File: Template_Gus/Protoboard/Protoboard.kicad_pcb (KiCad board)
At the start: 2 copper layers, 247 x 81.3 mm, 2 parts

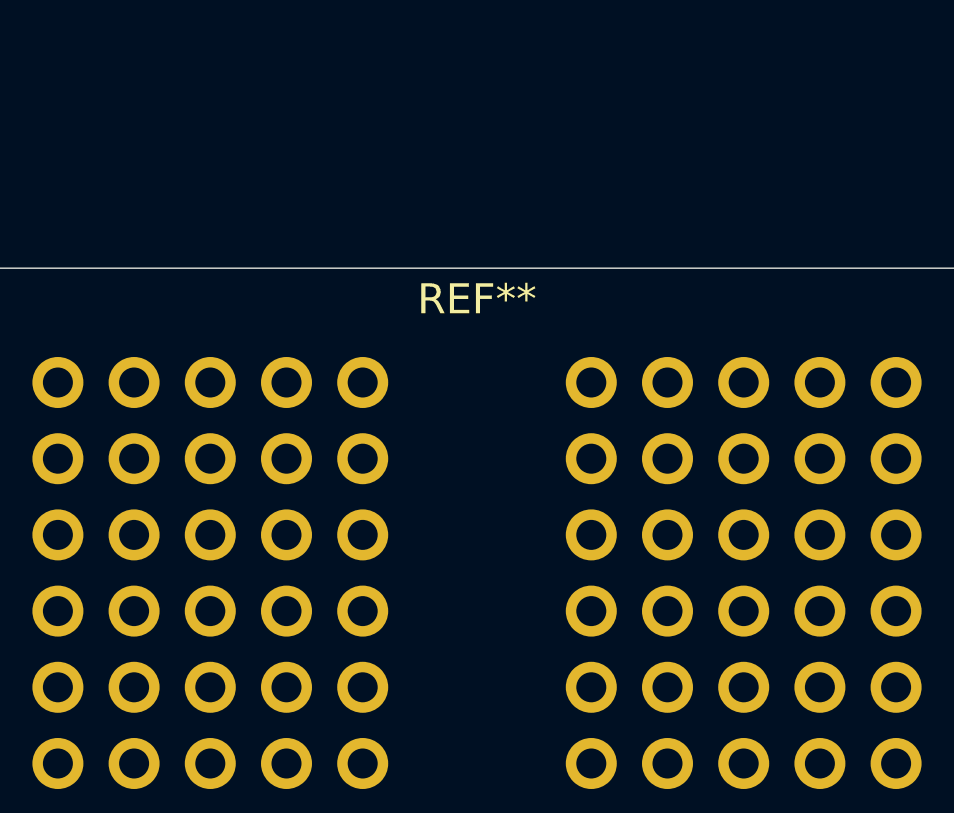
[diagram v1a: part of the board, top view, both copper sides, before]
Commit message: Add the Key
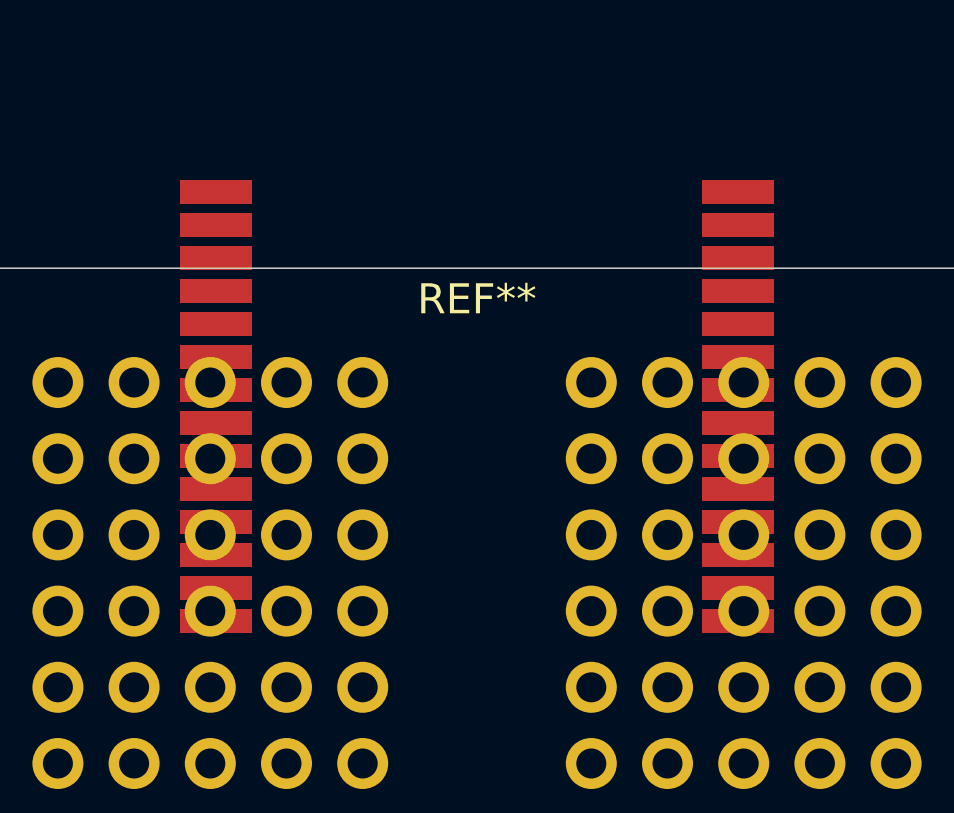
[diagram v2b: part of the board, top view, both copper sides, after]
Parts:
- added REF**: MS88SF2, Nordic_Module:MS88SF2, F.Cu at (49.5, 61.0)
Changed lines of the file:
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@@
     (tracks 0)
     (zones 0)
-    (modules 2)
+    (modules 3)
     (nets 1)
   )
@@
     (uvia_drill 0.1)
   )
+  (module Nordic_Module:MS88SF2 (layer F.Cu)
+    (at 49.53 60.96)
+    (fp_text reference REF** (at 0 -16.51) (layer F.Fab) hide
+      (effects (font (size 1 1) (thickness 0.15)))
+    )
+    (fp_text value MS88SF2 (at 0 10.795) (layer F.Fab) hide
+      (effects (font (size 1 1) (thickness 0.15)))
+    )
+    (fp_line (start -8.7 8.6868) (end 8.7 8.6868) (layer F.Fab) (width 0.12))
+    (fp_line (start -8.7 8.6868) (end -8.7 -14.5132) (layer F.Fab) (width 0.12))
+    (fp_line (start 8.7 8.6868) (end 8.7 -14.5132) (layer F.Fab) (width 0.12))
+    (fp_line (start -8.7 -14.5132) (end 8.7 -14.5132) (layer F.Fab) (width 0.12))
+    (fp_line (start -8.6868 -7.62) (end 8.6868 -7.62) (layer F.Fab) (width 0.12))
+    (fp_line (start 8.6868 -7.62) (end -8.6868 -14.5034) (layer F.Fab) (width 0.12))
+    (fp_line (start 8.6868 -14.5034) (end -8.6868 -7.62) (layer F.Fab) (width 0.12))
+    (pad 1 smd rect (at -8.7 -6.985) (size 2.4 0.8) (layers F.Cu F.Paste F.Mask))
+    (pad 2 smd rect (at -8.7 -5.885) (size 2.4 0.8) (layers F.Cu F.Paste F.Mask))
+    (pad 3 smd rect (at -8.7 -4.785) (size 2.4 0.8) (layers F.Cu F.Paste F.Mask))
+    (pad 4 smd rect (at -8.7 -3.685) (size 2.4 0.8) (layers F.Cu F.Paste F.Mask))
+    (pad 5 smd rect (at -8.7 -2.585) (size 2.4 0.8) (layers F.Cu F.Paste F.Mask))
+    (pad 6 smd rect (at -8.7 -1.485) (size 2.4 0.8) (layers F.Cu F.Paste F.Mask))
+    (pad 7 smd rect (at -8.7 -0.385) (size 2.4 0.8) (layers F.Cu F.Paste F.Mask))
+    (pad 8 smd rect (at -8.7 0.715) (size 2.4 0.8) (layers F.Cu F.Paste F.Mask))
+    (pad 9 smd rect (at -8.7 1.815) (size 2.4 0.8) (layers F.Cu F.Paste F.Mask))
+    (pad 10 smd rect (at -8.7 2.915) (size 2.4 0.8) (layers F.Cu F.Paste F.Mask))
+    (pad 11 smd rect (at -8.7 4.015) (size 2.4 0.8) (layers F.Cu F.Paste F.Mask))
+    (pad 12 smd rect (at -8.7 5.115) (size 2.4 0.8) (layers F.Cu F.Paste F.Mask))
+    (pad 13 smd rect (at -8.7 6.215) (size 2.4 0.8) (layers F.Cu F.Paste F.Mask))
+    (pad 14 smd rect (at -8.7 7.315) (size 2.4 0.8) (layers F.Cu F.Paste F.Mask))
+    (pad 28 smd rect (at 8.7 -6.985) (size 2.4 0.8) (layers F.Cu F.Paste F.Mask))
+    (pad 27 smd rect (at 8.7 -5.885) (size 2.4 0.8) (layers F.Cu F.Paste F.Mask))
+    (pad 26 smd rect (at 8.7 -4.785) (size 2.4 0.8) (layers F.Cu F.Paste F.Mask))
+    (pad 25 smd rect (at 8.7 -3.685) (size 2.4 0.8) (layers F.Cu F.Paste F.Mask))
+    (pad 24 smd rect (at 8.7 -2.585) (size 2.4 0.8) (layers F.Cu F.Paste F.Mask))
+    (pad 23 smd rect (at 8.7 -1.485) (size 2.4 0.8) (layers F.Cu F.Paste F.Mask))
+    (pad 22 smd rect (at 8.7 -0.385) (size 2.4 0.8) (layers F.Cu F.Paste F.Mask))
+    (pad 21 smd rect (at 8.7 0.715) (size 2.4 0.8) (layers F.Cu F.Paste F.Mask))
+    (pad 20 smd rect (at 8.7 1.815) (size 2.4 0.8) (layers F.Cu F.Paste F.Mask))
+    (pad 19 smd rect (at 8.7 2.915) (size 2.4 0.8) (layers F.Cu F.Paste F.Mask))
+    (pad 18 smd rect (at 8.7 4.015) (size 2.4 0.8) (layers F.Cu F.Paste F.Mask))
+    (pad 17 smd rect (at 8.7 5.115) (size 2.4 0.8) (layers F.Cu F.Paste F.Mask))
+    (pad 16 smd rect (at 8.7 6.215) (size 2.4 0.8) (layers F.Cu F.Paste F.Mask))
+    (pad 15 smd rect (at 8.7 7.315) (size 2.4 0.8) (layers F.Cu F.Paste F.Mask))
+  )
   (module Protoboard:Breadboard_Friendly_Template_800 (layer F.Cu)

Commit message: update
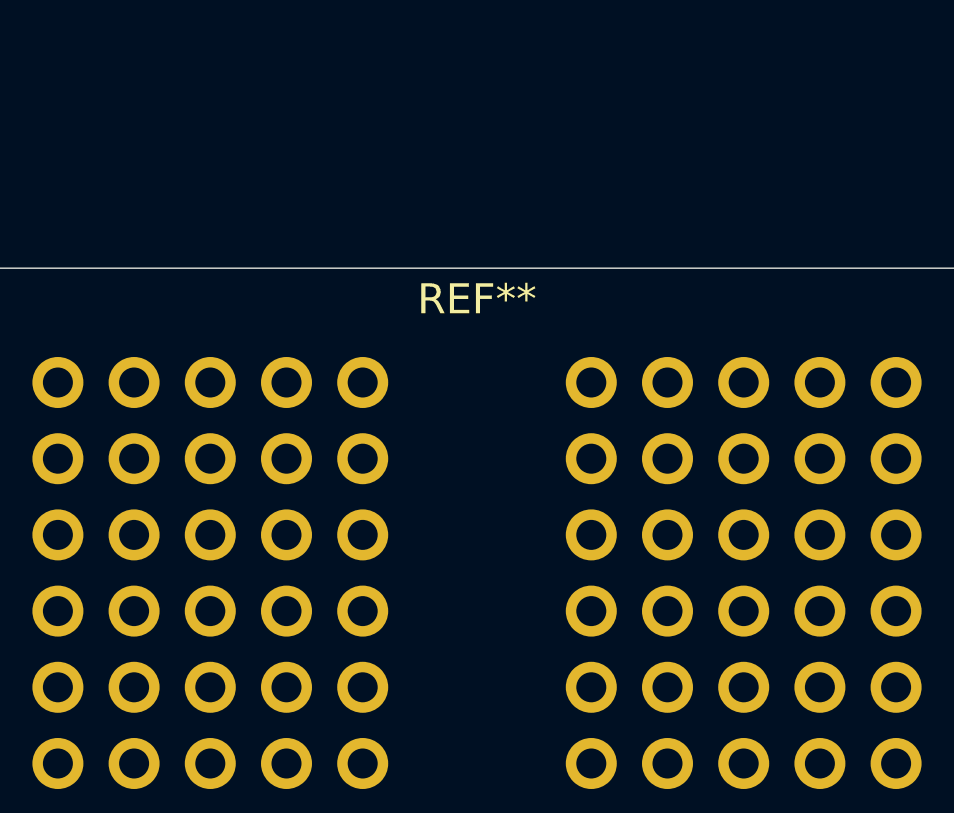
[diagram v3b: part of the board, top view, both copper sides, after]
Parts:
- removed the REF** at (49.5, 61.0)
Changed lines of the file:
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@@
-(kicad_pcb (version 20171130) (host pcbnew 5.1.5-52549c5~84~ubuntu18.04.1)
+(kicad_pcb (version 20171130) (host pcbnew "(5.1.9-0-10_14)")
   (general
     (thickness 1.6)
-    (drawings 33)
+    (drawings 37)
     (tracks 0)
     (zones 0)
-    (modules 3)
+    (modules 2)
     (nets 1)
   )
@@
     (uvia_dia 0.3)
     (uvia_drill 0.1)
-  )
-  (module Nordic_Module:MS88SF2 (layer F.Cu)
-    (at 49.53 60.96)
-    (fp_text reference REF** (at 0 -16.51) (layer F.Fab) hide
-      (effects (font (size 1 1) (thickness 0.15)))
-    )
-    (fp_text value MS88SF2 (at 0 10.795) (layer F.Fab) hide
-      (effects (font (size 1 1) (thickness 0.15)))
-    )
-    (fp_line (start -8.7 8.6868) (end 8.7 8.6868) (layer F.Fab) (width 0.12))
-    (fp_line (start -8.7 8.6868) (end -8.7 -14.5132) (layer F.Fab) (width 0.12))
-    (fp_line (start 8.7 8.6868) (end 8.7 -14.5132) (layer F.Fab) (width 0.12))
-    (fp_line (start -8.7 -14.5132) (end 8.7 -14.5132) (layer F.Fab) (width 0.12))
-    (fp_line (start -8.6868 -7.62) (end 8.6868 -7.62) (layer F.Fab) (width 0.12))
-    (fp_line (start 8.6868 -7.62) (end -8.6868 -14.5034) (layer F.Fab) (width 0.12))
-    (fp_line (start 8.6868 -14.5034) (end -8.6868 -7.62) (layer F.Fab) (width 0.12))
-    (pad 1 smd rect (at -8.7 -6.985) (size 2.4 0.8) (layers F.Cu F.Paste F.Mask))
-    (pad 2 smd rect (at -8.7 -5.885) (size 2.4 0.8) (layers F.Cu F.Paste F.Mask))
-    (pad 3 smd rect (at -8.7 -4.785) (size 2.4 0.8) (layers F.Cu F.Paste F.Mask))
-    (pad 4 smd rect (at -8.7 -3.685) (size 2.4 0.8) (layers F.Cu F.Paste F.Mask))
-    (pad 5 smd rect (at -8.7 -2.585) (size 2.4 0.8) (layers F.Cu F.Paste F.Mask))
-    (pad 6 smd rect (at -8.7 -1.485) (size 2.4 0.8) (layers F.Cu F.Paste F.Mask))
-    (pad 7 smd rect (at -8.7 -0.385) (size 2.4 0.8) (layers F.Cu F.Paste F.Mask))
-    (pad 8 smd rect (at -8.7 0.715) (size 2.4 0.8) (layers F.Cu F.Paste F.Mask))
-    (pad 9 smd rect (at -8.7 1.815) (size 2.4 0.8) (layers F.Cu F.Paste F.Mask))
-    (pad 10 smd rect (at -8.7 2.915) (size 2.4 0.8) (layers F.Cu F.Paste F.Mask))
-    (pad 11 smd rect (at -8.7 4.015) (size 2.4 0.8) (layers F.Cu F.Paste F.Mask))
-    (pad 12 smd rect (at -8.7 5.115) (size 2.4 0.8) (layers F.Cu F.Paste F.Mask))
-    (pad 13 smd rect (at -8.7 6.215) (size 2.4 0.8) (layers F.Cu F.Paste F.Mask))
-    (pad 14 smd rect (at -8.7 7.315) (size 2.4 0.8) (layers F.Cu F.Paste F.Mask))
-    (pad 28 smd rect (at 8.7 -6.985) (size 2.4 0.8) (layers F.Cu F.Paste F.Mask))
-    (pad 27 smd rect (at 8.7 -5.885) (size 2.4 0.8) (layers F.Cu F.Paste F.Mask))
-    (pad 26 smd rect (at 8.7 -4.785) (size 2.4 0.8) (layers F.Cu F.Paste F.Mask))
-    (pad 25 smd rect (at 8.7 -3.685) (size 2.4 0.8) (layers F.Cu F.Paste F.Mask))
-    (pad 24 smd rect (at 8.7 -2.585) (size 2.4 0.8) (layers F.Cu F.Paste F.Mask))
-    (pad 23 smd rect (at 8.7 -1.485) (size 2.4 0.8) (layers F.Cu F.Paste F.Mask))
-    (pad 22 smd rect (at 8.7 -0.385) (size 2.4 0.8) (layers F.Cu F.Paste F.Mask))
-    (pad 21 smd rect (at 8.7 0.715) (size 2.4 0.8) (layers F.Cu F.Paste F.Mask))
-    (pad 20 smd rect (at 8.7 1.815) (size 2.4 0.8) (layers F.Cu F.Paste F.Mask))
-    (pad 19 smd rect (at 8.7 2.915) (size 2.4 0.8) (layers F.Cu F.Paste F.Mask))
-    (pad 18 smd rect (at 8.7 4.015) (size 2.4 0.8) (layers F.Cu F.Paste F.Mask))
-    (pad 17 smd rect (at 8.7 5.115) (size 2.4 0.8) (layers F.Cu F.Paste F.Mask))
-    (pad 16 smd rect (at 8.7 6.215) (size 2.4 0.8) (layers F.Cu F.Paste F.Mask))
-    (pad 15 smd rect (at 8.7 7.315) (size 2.4 0.8) (layers F.Cu F.Paste F.Mask))
   )
   (module Protoboard:Breadboard_Friendly_Template_800 (layer F.Cu)
@@
     (pad 22 thru_hole oval (at -6.35 16.51) (size 1.7 1.7) (drill 1) (layers *.Cu *.Mask))
   )
+  (dimension 22.86 (width 0.15) (layer Dwgs.User)
+    (gr_text "22.860 mm" (at 49.53 151.16) (layer Dwgs.User)
+      (effects (font (size 1 1) (thickness 0.15)))
+    )
+    (feature1 (pts (xy 38.1 133.985) (xy 38.1 150.446421)))
+    (feature2 (pts (xy 60.96 133.985) (xy 60.96 150.446421)))
+    (crossbar (pts (xy 60.96 149.86) (xy 38.1 149.86)))
+    (arrow1a (pts (xy 38.1 149.86) (xy 39.226504 149.273579)))
+    (arrow1b (pts (xy 38.1 149.86) (xy 39.226504 150.446421)))
+    (arrow2a (pts (xy 60.96 149.86) (xy 59.833496 149.273579)))
+    (arrow2b (pts (xy 60.96 149.86) (xy 59.833496 150.446421)))
+  )
+  (dimension 17.78 (width 0.15) (layer Dwgs.User)
+    (gr_text "17.780 mm" (at 49.53 147.985) (layer Dwgs.User)
+      (effects (font (size 1 1) (thickness 0.15)))
+    )
+    (feature1 (pts (xy 40.64 133.985) (xy 40.64 147.271421)))
+    (feature2 (pts (xy 58.42 133.985) (xy 58.42 147.271421)))
+    (crossbar (pts (xy 58.42 146.685) (xy 40.64 146.685)))
+    (arrow1a (pts (xy 40.64 146.685) (xy 41.766504 146.098579)))
+    (arrow1b (pts (xy 40.64 146.685) (xy 41.766504 147.271421)))
+    (arrow2a (pts (xy 58.42 146.685) (xy 57.293496 146.098579)))
+    (arrow2b (pts (xy 58.42 146.685) (xy 57.293496 147.271421)))
+  )
+  (dimension 12.7 (width 0.15) (layer Dwgs.User)
+    (gr_text "12.700 mm" (at 49.53 144.81) (layer Dwgs.User)
+      (effects (font (size 1 1) (thickness 0.15)))
+    )
+    (feature1 (pts (xy 55.88 133.985) (xy 55.88 144.096421)))
+    (feature2 (pts (xy 43.18 133.985) (xy 43.18 144.096421)))
+    (crossbar (pts (xy 43.18 143.51) (xy 55.88 143.51)))
+    (arrow1a (pts (xy 55.88 143.51) (xy 54.753496 144.096421)))
+    (arrow1b (pts (xy 55.88 143.51) (xy 54.753496 142.923579)))
+    (arrow2a (pts (xy 43.18 143.51) (xy 44.306504 144.096421)))
+    (arrow2b (pts (xy 43.18 143.51) (xy 44.306504 142.923579)))
+  )
+  (dimension 7.62 (width 0.15) (layer Dwgs.User)
+    (gr_text "7.620 mm" (at 49.53 141.635) (layer Dwgs.User)
+      (effects (font (size 1 1) (thickness 0.15)))
+    )
+    (feature1 (pts (xy 53.34 133.985) (xy 53.34 140.921421)))
+    (feature2 (pts (xy 45.72 133.985) (xy 45.72 140.921421)))
+    (crossbar (pts (xy 45.72 140.335) (xy 53.34 140.335)))
+    (arrow1a (pts (xy 53.34 140.335) (xy 52.213496 140.921421)))
+    (arrow1b (pts (xy 53.34 140.335) (xy 52.213496 139.748579)))
+    (arrow2a (pts (xy 45.72 140.335) (xy 46.846504 140.921421)))
+    (arrow2b (pts (xy 45.72 140.335) (xy 46.846504 139.748579)))
+  )
   (dimension 22.86 (width 0.15) (layer F.Fab)
